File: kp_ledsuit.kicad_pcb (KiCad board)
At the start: 2 copper layers, 63.1 x 36.5 mm, 79 parts, among them IC1 MP2359DJ-LF-Z, J1 USB_B_Mini, J2 SWD, J3 Conn_01x04_MountingPin, J4 SK9822, Q1 AO3401A, Q2 BC818, SW1 SW_SPDT, U1 STM32F103C8Tx, U2 USBLC6-2P6, U3 LSM6DS3, Y1 12MHz

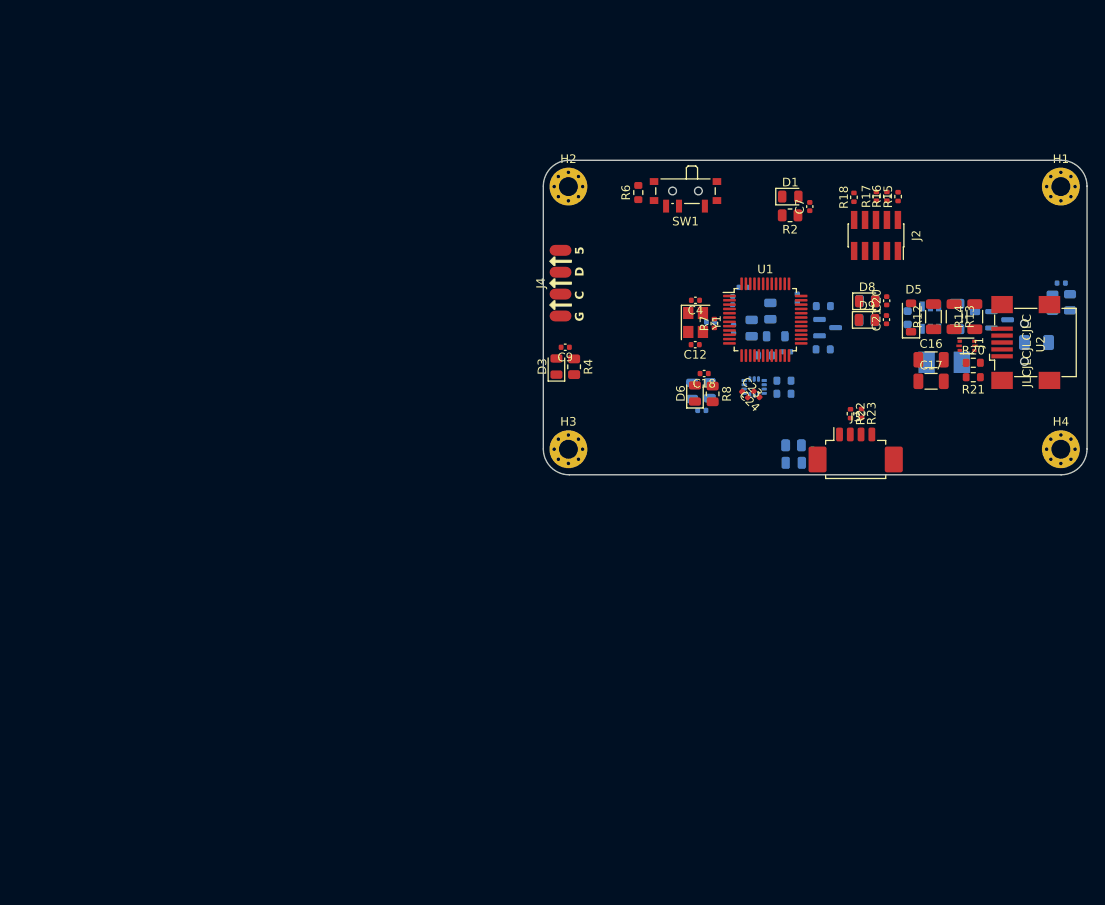
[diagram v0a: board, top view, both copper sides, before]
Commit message: WIP first proto layout: 1 face
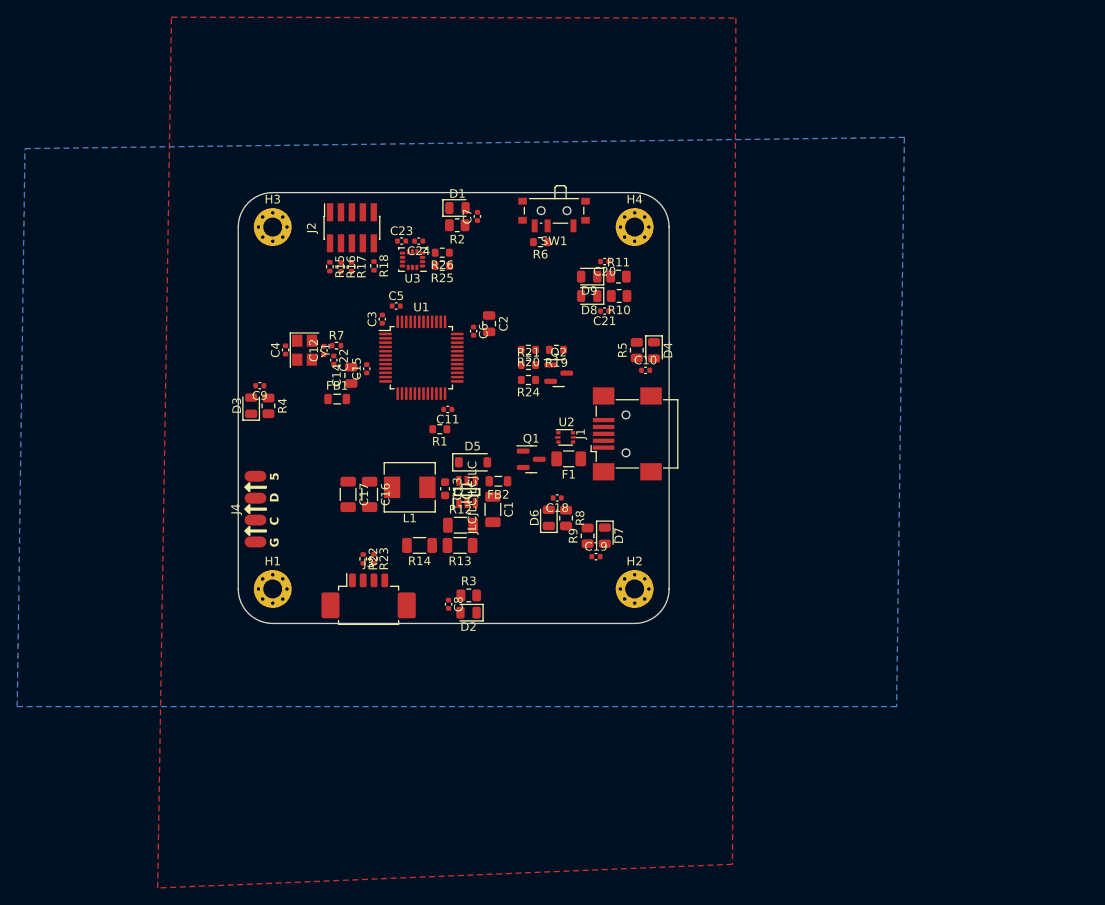
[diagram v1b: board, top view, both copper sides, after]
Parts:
- C1, C10, C11, C13, C14, C15, C19, C2, C22, C3, C5, C6, C8, D2, D4, D7, F1, FB1, FB2, IC1, L1, Q1, Q2, R1, R10, R11, R19, R24, R25, R26, R3, R5, R9, U3: moved to F.Cu
- moved H1 102.7 mm to (122.0, 123.0)
- moved R14 69.7 mm to (139.0, 118.0), turned to 180 degrees
- moved C17 68.9 mm to (130.8, 112.0), turned to -90 degrees
- moved C16 67.0 mm to (133.2, 112.0), turned to -90 degrees
- moved R15 66.4 mm to (128.6, 85.6), turned to -90 degrees
- moved R16 63.9 mm to (129.9, 85.6), turned to -90 degrees
- moved L1 63.7 mm to (137.9, 111.2)
- moved R13 63.2 mm to (143.7, 118.0), turned to 180 degrees
- moved R17 61.4 mm to (131.2, 85.6), turned to -90 degrees
- moved J2 60.8 mm to (131.2, 81.1), turned to 90 degrees
- moved R12 60.0 mm to (143.8, 115.6), turned to 0 degrees
- moved R23 59.0 mm to (133.8, 119.5)
- moved R22 59.0 mm to (132.5, 119.5)
- moved J3 59.0 mm to (133.1, 124.4)
- moved FB2 58.4 mm to (148.2, 110.5), turned to 180 degrees
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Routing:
- added copper zone on In1.Cu, net +3.3V
- added copper zone on B.Cu, net GND
- added copper zone on F.Cu, net GND
- added copper zone on In2.Cu, net GND
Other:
- board size 63.1 x 36.5 mm -> 50 x 50 mm
- copper layers 2 -> 4

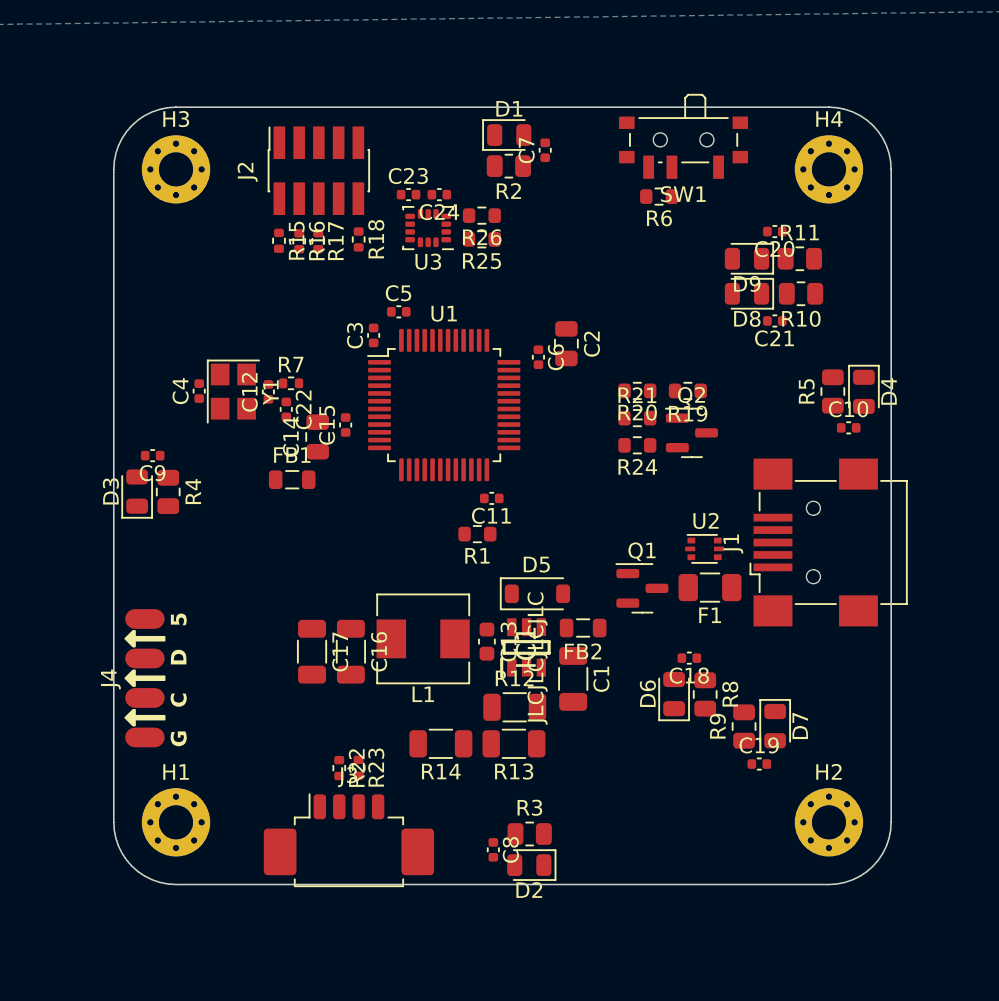
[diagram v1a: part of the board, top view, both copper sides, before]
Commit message: pxm test logo
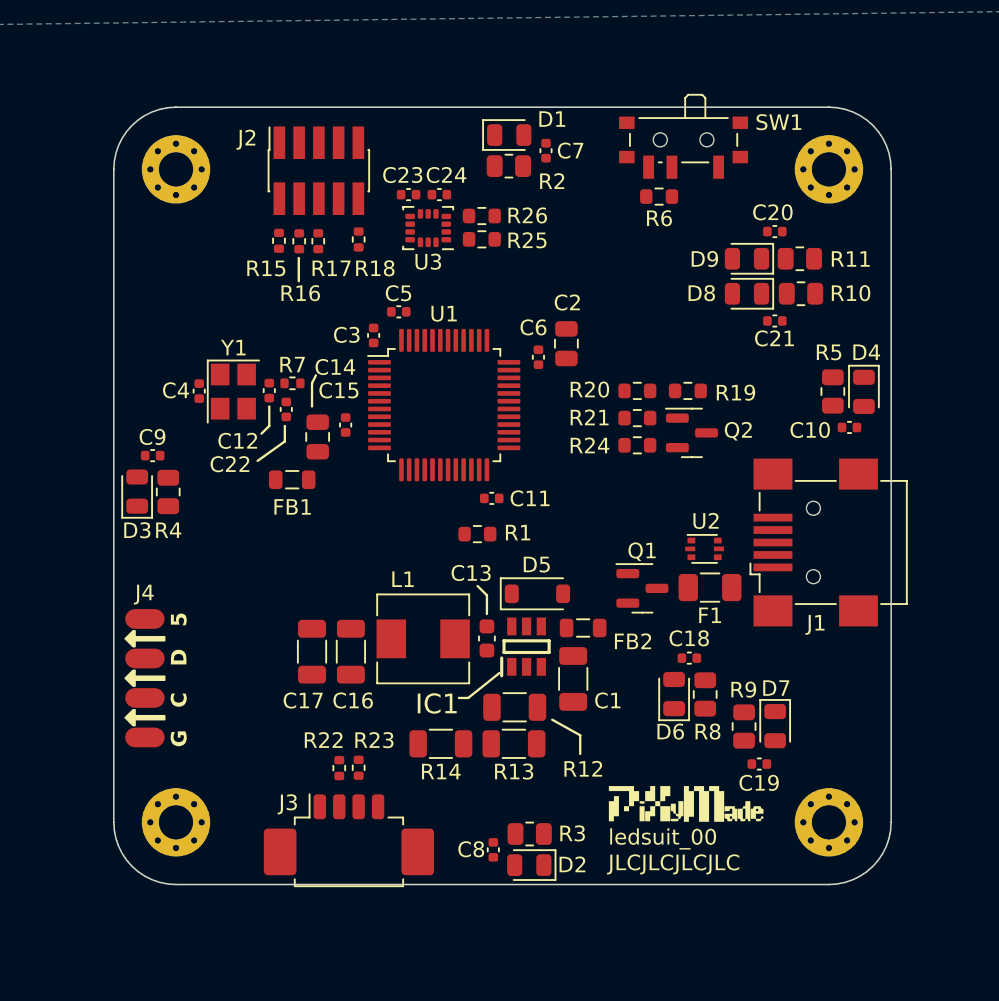
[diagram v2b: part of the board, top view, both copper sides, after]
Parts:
- added G***: LOGO, homemade_footprints:pxm_testlogo_v1, F.Cu at (154.8, 121.8)
- moved C13 0.20 mm to (142.0, 111.2)
- moved C12 0.10 mm to (128.0, 95.2)
- moved R7 0.09 mm to (129.5, 94.8)
- moved C7 0.06 mm to (145.8, 79.8)
- moved C10 0.06 mm to (165.3, 97.6)
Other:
- board text added: "ledsuit_00"
